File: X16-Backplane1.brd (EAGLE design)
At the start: 131.3 x 110.3 mm, 26 parts, among them J1 CONN_PXC-8-RA-1778683, J12 282837-3, J13 282837-3, J2 CONN_ET60S-D04-3-08-D04-X-R1-S, J3 HTST-110-04-L-D-RA, J4 CLT-110-01-F-D, U2 TRANS_ULN2003AD

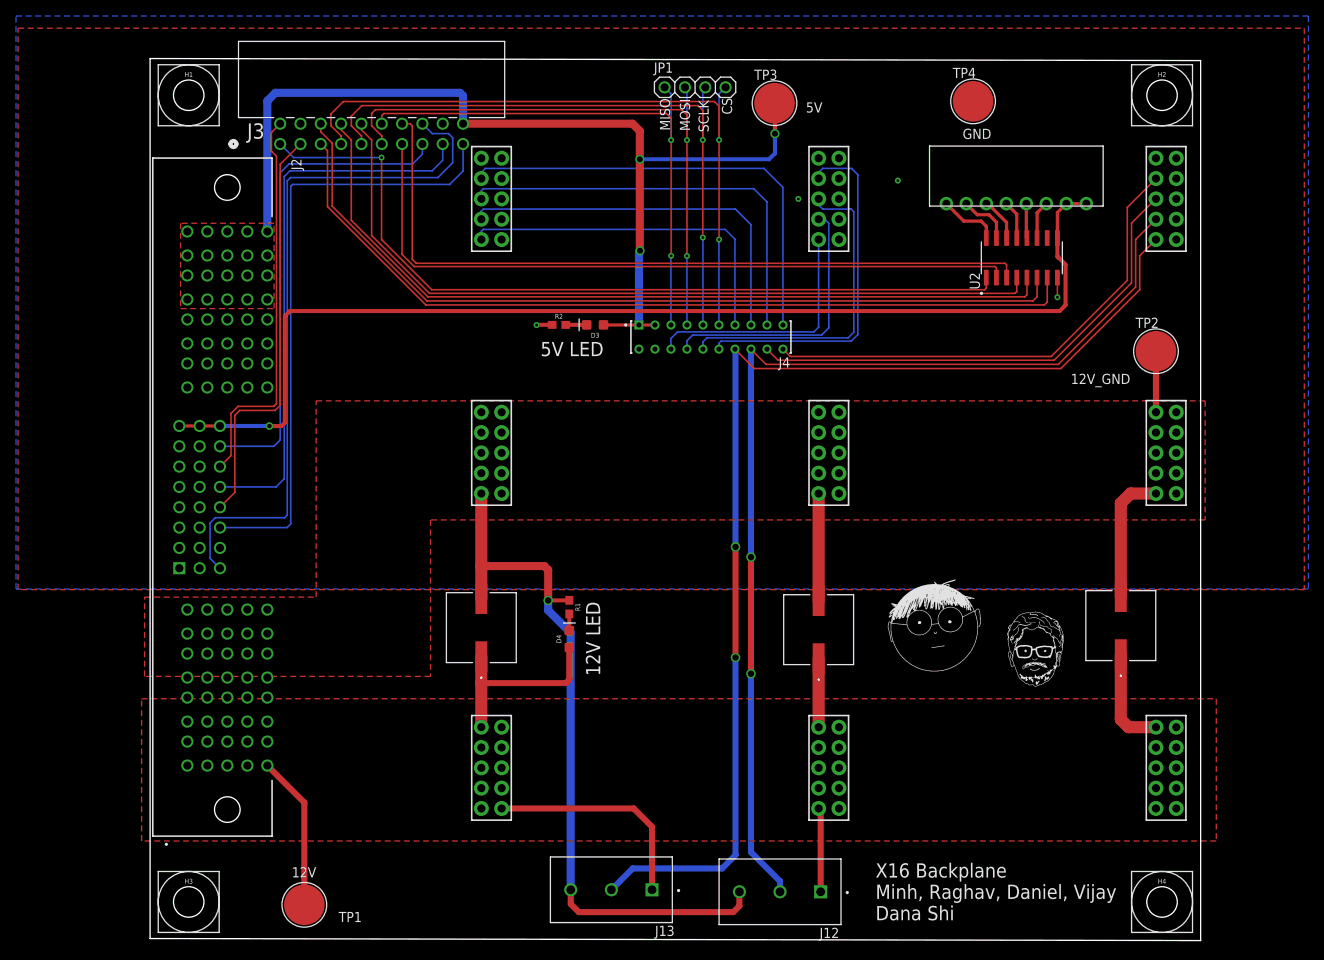
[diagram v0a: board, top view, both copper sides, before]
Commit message: Minh Update 4
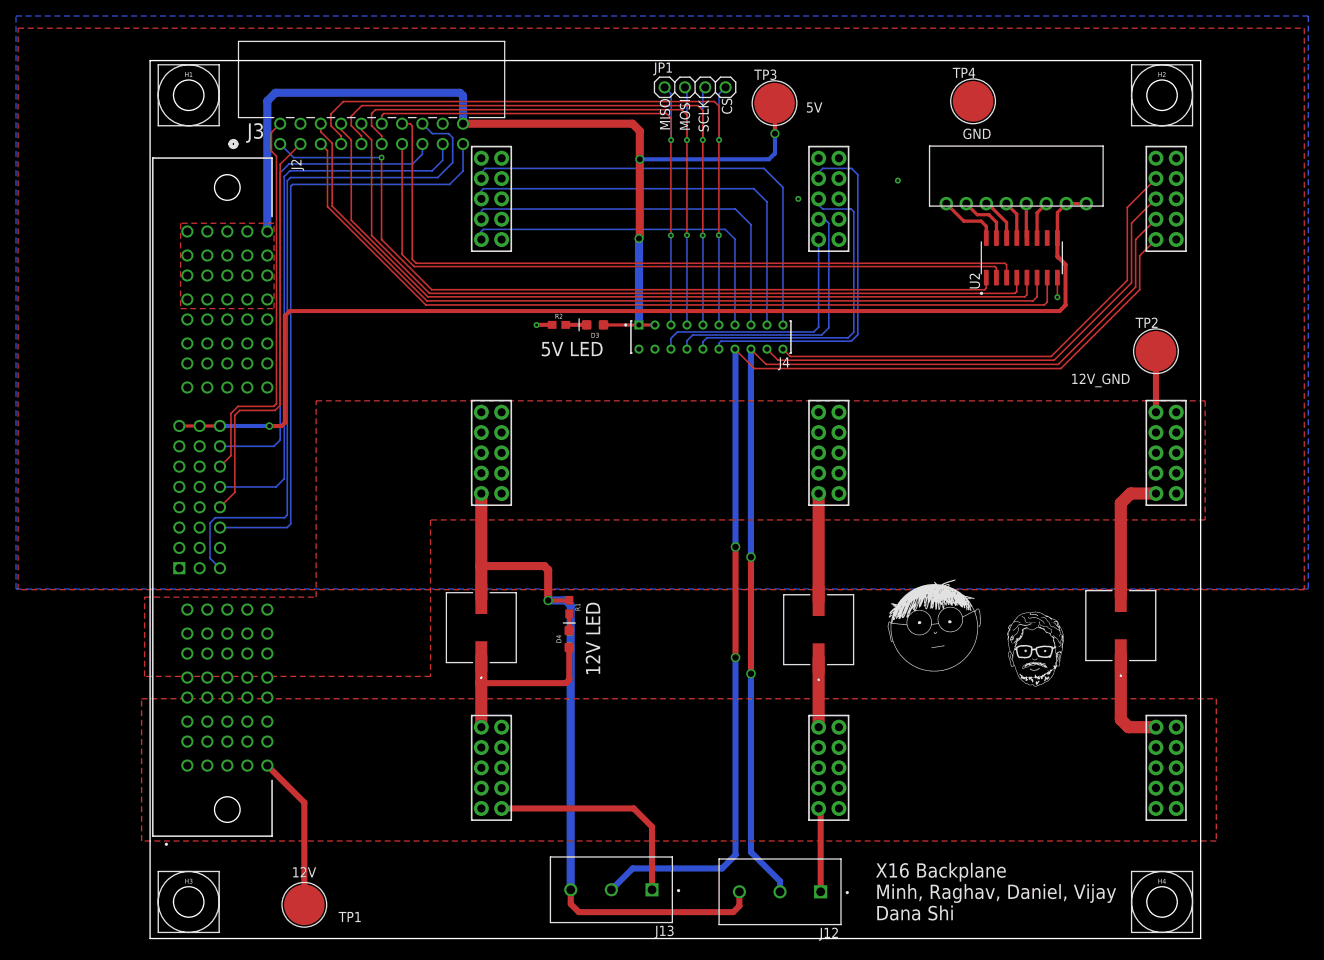
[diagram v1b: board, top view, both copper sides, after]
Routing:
- net 12V_GND: track 128.5 -> 129.8 mm
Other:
- board size 131.3 x 110.3 mm -> 131.3 x 109.7 mm
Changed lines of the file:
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@@
 <board>
 <plain>
-<wire x1="0" y1="0" x2="131.318" y2="-0.254" width="0" layer="20"/>
-<wire x1="131.318" y1="-0.254" x2="131.318" y2="109.746" width="0" layer="20"/>
-<wire x1="131.318" y1="109.746" x2="0" y2="110" width="0" layer="20"/>
-<wire x1="0" y1="110" x2="0" y2="0" width="0" layer="20"/>
+<wire x1="0" y1="0" x2="131.318" y2="0" width="0" layer="20"/>
+<wire x1="131.318" y1="0" x2="131.318" y2="109.746" width="0" layer="20"/>
+<wire x1="131.318" y1="109.746" x2="0" y2="109.746" width="0" layer="20"/>
+<wire x1="0" y1="109.746" x2="0" y2="0" width="0" layer="20"/>
 <polygon width="0.4064" layer="29">
 <vertex x="23.368" y="56.388"/>
@@
 <wire x1="41.402" y1="55.626" x2="41.402" y2="46.5582" width="1.524" layer="1"/>
 <wire x1="125.73" y1="65.786" x2="125.73" y2="73.406" width="0.762" layer="1"/>
-<wire x1="52.578" y1="6.096" x2="52.578" y2="38.2016" width="1.016" layer="16"/>
-<wire x1="49.7586" y1="41.021" x2="49.7586" y2="42.2656" width="1.016" layer="16"/>
+<wire x1="52.578" y1="6.096" x2="52.578" y2="41.6306" width="1.016" layer="16"/>
 <via x="49.7586" y="42.2656" extent="1-16" drill="0.8"/>
-<wire x1="52.578" y1="38.2016" x2="49.7586" y2="41.021" width="1.016" layer="16"/>
+<wire x1="52.578" y1="41.6306" x2="51.943" y2="42.2656" width="1.016" layer="16"/>
+<wire x1="49.7586" y1="42.2656" x2="51.943" y2="42.2656" width="1.016" layer="16"/>
 <wire x1="49.7586" y1="42.2656" x2="49.7586" y2="46.0756" width="1.016" layer="1"/>
 <wire x1="49.7586" y1="46.0756" x2="49.276" y2="46.5582" width="1.016" layer="1"/>
@@
 <wire x1="61.214" y1="100.9396" x2="61.214" y2="97.409" width="1.016" layer="1"/>
 <via x="61.214" y="97.409" extent="1-16" drill="0.75"/>
-<wire x1="61.214" y1="97.409" x2="61.214" y2="86.0044" width="1.016" layer="1"/>
-<wire x1="61.214" y1="86.0044" x2="61.2394" y2="85.979" width="1.016" layer="1"/>
-<via x="61.2394" y="85.979" extent="1-16" drill="0.75"/>
-<wire x1="61.2394" y1="85.979" x2="61.1124" y2="85.852" width="1.016" layer="16"/>
-<wire x1="61.1124" y1="85.852" x2="61.1124" y2="76.7024" width="1.016" layer="16"/>
+<wire x1="61.214" y1="97.409" x2="61.214" y2="87.6046" width="1.016" layer="1"/>
+<wire x1="61.214" y1="87.6046" x2="61.1124" y2="87.503" width="1.016" layer="1"/>
+<via x="61.1124" y="87.503" extent="1-16" drill="0.75"/>
+<wire x1="61.1124" y1="87.503" x2="61.1124" y2="76.7024" width="1.016" layer="16"/>
 <wire x1="61.1124" y1="76.7024" x2="61.104" y2="76.694" width="1.016" layer="16"/>
 <wire x1="61.214" y1="97.409" x2="77.3684" y2="97.409" width="0.508" layer="16"/>
@@
 <contactref element="J4" pad="05"/>
 <contactref element="J3" pad="12"/>
-<wire x1="65.104" y1="76.694" x2="65.104" y2="85.3224" width="0.2032" layer="16"/>
-<wire x1="65.104" y1="85.3224" x2="65.1256" y2="85.344" width="0.2032" layer="16"/>
-<via x="65.1256" y="85.344" extent="1-16" drill="0.35"/>
-<wire x1="65.1256" y1="85.344" x2="65.1256" y2="99.7966" width="0.2032" layer="1"/>
+<wire x1="65.104" y1="76.694" x2="65.104" y2="87.8802" width="0.2032" layer="16"/>
+<wire x1="65.104" y1="87.8802" x2="65.1002" y2="87.884" width="0.2032" layer="16"/>
+<via x="65.1002" y="87.884" extent="1-16" drill="0.35"/>
+<wire x1="65.1002" y1="99.7712" x2="65.1256" y2="99.7966" width="0.2032" layer="1"/>
+<wire x1="65.1002" y1="99.7712" x2="65.1002" y2="87.884" width="0.2032" layer="1"/>
 <wire x1="65.1256" y1="99.7966" x2="65.1256" y2="102.5398" width="0.2032" layer="1"/>
 <wire x1="65.1256" y1="102.5398" x2="64.5414" y2="103.124" width="0.2032" layer="1"/>
@@
 <contactref element="J4" pad="07"/>
 <contactref element="J3" pad="11"/>
-<wire x1="67.104" y1="76.694" x2="67.104" y2="85.3158" width="0.2032" layer="16"/>
-<wire x1="67.104" y1="85.3158" x2="67.1068" y2="85.3186" width="0.2032" layer="16"/>
-<via x="67.1068" y="85.3186" extent="1-16" drill="0.35"/>
-<wire x1="67.1068" y1="85.3186" x2="67.1068" y2="99.7966" width="0.2032" layer="1"/>
+<wire x1="67.104" y1="76.694" x2="67.104" y2="87.9066" width="0.2032" layer="16"/>
+<wire x1="67.104" y1="87.9066" x2="67.1068" y2="87.9094" width="0.2032" layer="16"/>
+<via x="67.1068" y="87.9094" extent="1-16" drill="0.35"/>
+<wire x1="67.1068" y1="87.9094" x2="67.1068" y2="99.7966" width="0.2032" layer="1"/>
 <wire x1="67.1068" y1="99.7966" x2="67.1068" y2="102.9462" width="0.2032" layer="1"/>
 <wire x1="67.1068" y1="102.9462" x2="66.4464" y2="103.6066" width="0.2032" layer="1"/>
@@
 <contactref element="J4" pad="09"/>
 <contactref element="J3" pad="9"/>
-<wire x1="69.104" y1="76.694" x2="69.104" y2="87.614" width="0.2032" layer="16"/>
-<wire x1="69.104" y1="87.614" x2="69.088" y2="87.63" width="0.2032" layer="16"/>
-<via x="69.088" y="87.63" extent="1-16" drill="0.35"/>
-<wire x1="69.088" y1="87.63" x2="69.088" y2="99.822" width="0.2032" layer="1"/>
+<wire x1="69.104" y1="76.694" x2="69.104" y2="87.868" width="0.2032" layer="16"/>
+<wire x1="69.104" y1="87.868" x2="69.088" y2="87.884" width="0.2032" layer="16"/>
+<via x="69.088" y="87.884" extent="1-16" drill="0.35"/>
+<wire x1="69.088" y1="87.884" x2="69.088" y2="99.822" width="0.2032" layer="1"/>
 <wire x1="69.088" y1="99.822" x2="69.088" y2="103.505" width="0.2032" layer="1"/>
 <wire x1="69.088" y1="103.505" x2="68.4784" y2="104.1146" width="0.2032" layer="1"/>
@@
 <contactref element="J4" pad="11"/>
 <contactref element="J3" pad="7"/>
-<wire x1="71.104" y1="76.694" x2="71.104" y2="87.36" width="0.2032" layer="16"/>
-<wire x1="71.104" y1="87.36" x2="71.12" y2="87.376" width="0.2032" layer="16"/>
-<via x="71.12" y="87.376" extent="1-16" drill="0.35"/>
-<wire x1="71.12" y1="87.376" x2="71.12" y2="99.822" width="0.2032" layer="1"/>
+<wire x1="71.104" y1="76.694" x2="71.104" y2="87.9" width="0.2032" layer="16"/>
+<wire x1="71.104" y1="87.9" x2="71.0946" y2="87.9094" width="0.2032" layer="16"/>
+<via x="71.0946" y="87.9094" extent="1-16" drill="0.35"/>
+<wire x1="71.0946" y1="99.7966" x2="71.12" y2="99.822" width="0.2032" layer="1"/>
+<wire x1="71.0946" y1="99.7966" x2="71.0946" y2="87.9094" width="0.2032" layer="1"/>
 <wire x1="71.12" y1="99.822" x2="71.12" y2="104.0384" width="0.2032" layer="1"/>
 <wire x1="70.5358" y1="104.6226" x2="71.12" y2="104.0384" width="0.2032" layer="1"/>
